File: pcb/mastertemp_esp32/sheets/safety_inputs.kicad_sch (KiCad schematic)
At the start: 0 parts

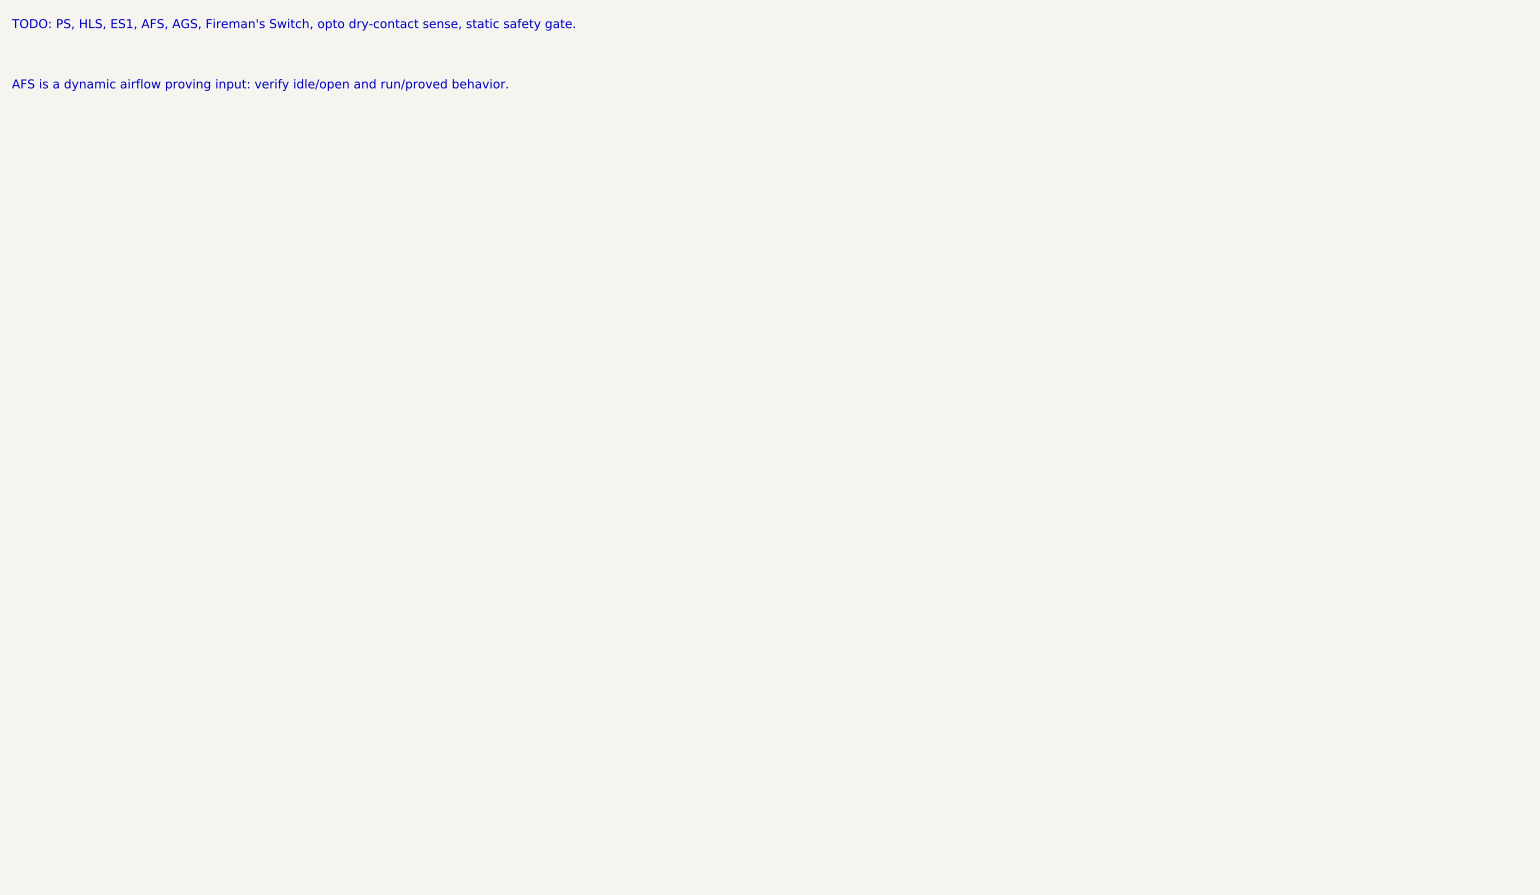
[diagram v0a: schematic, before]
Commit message: Bump
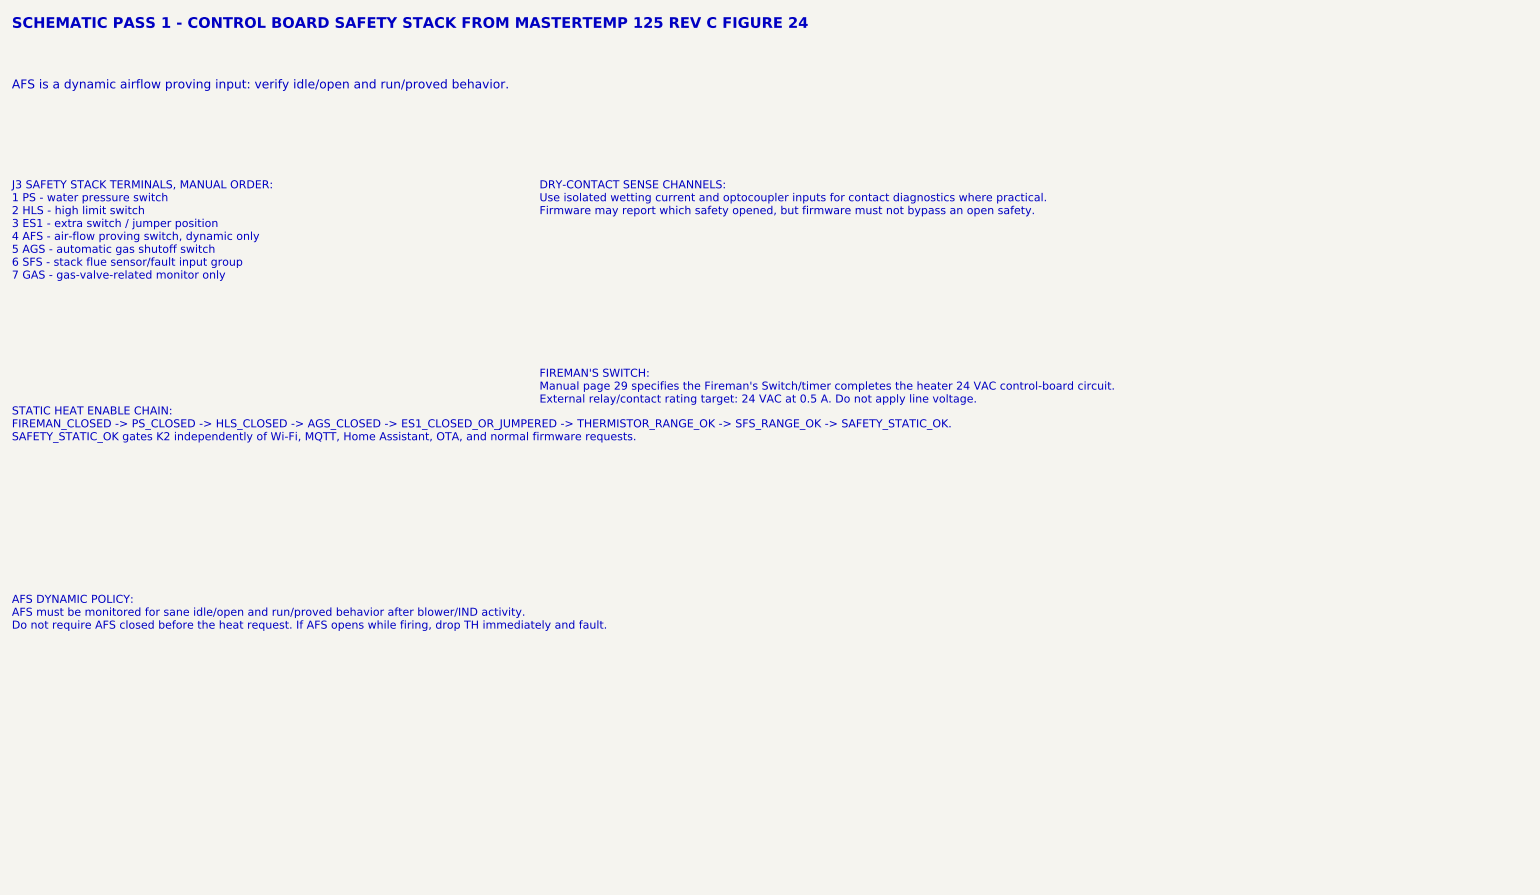
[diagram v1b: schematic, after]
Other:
- note added: "AFS DYNAMIC POLICY: AFS must be monitored for sane idle/open and run/proved behavior after blower/IND activity. Do not require AFS closed before the heat request. If AFS opens while firing, drop TH immediately and fault."
- note added: "DRY-CONTACT SENSE CHANNELS: Use isolated wetting current and optocoupler inputs for contact diagnostics where practical. Firmware may report which safety opened, but firmware must not bypass an open safety."
- note added: "FIREMAN'S SWITCH: Manual page 29 specifies the Fireman's Switch/timer completes the heater 24 VAC control-board circuit. External relay/contact rating target: 24 VAC at 0.5 A. Do not apply line voltage."
- note added: "J3 SAFETY STACK TERMINALS, MANUAL ORDER: 1 PS - water pressure switch 2 HLS - high limit switch 3 ES1 - extra switch / jumper position 4 AFS - air-flow proving switch, dynamic only 5 AGS - automatic gas shutoff switch 6 SFS - stack flue sensor/fault input group 7 GAS - gas-valve-related monitor only"
- note added: "SCHEMATIC PASS 1 - CONTROL BOARD SAFETY STACK FROM MASTERTEMP 125 REV C FIGURE 24"
- note added: "STATIC HEAT ENABLE CHAIN: FIREMAN_CLOSED -> PS_CLOSED -> HLS_CLOSED -> AGS_CLOSED -> ES1_CLOSED_OR_JUMPERED -> THERMISTOR_RANGE_OK -> SFS_RANGE_OK -> SAFETY_STATIC_OK. SAFETY_STATIC_OK gates K2 independently of Wi-Fi, MQTT, Home Assistant, OTA, and normal firmware requests."
- note removed: "TODO: PS, HLS, ES1, AFS, AGS, Fireman's Switch, opto dry-contact sense, static safety gate."
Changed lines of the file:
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@@
     (comment 1 "Safety switches are sensed and participate in hardware gating where appropriate.")
   )
-  (text "TODO: PS, HLS, ES1, AFS, AGS, Fireman's Switch, opto dry-contact sense, static safety gate."
+  (text "SCHEMATIC PASS 1 - CONTROL BOARD SAFETY STACK FROM MASTERTEMP 125 REV C FIGURE 24"
     (at 25.4 25.4 0)
-    (effects (font (size 1.5 1.5)) (justify left bottom))
+    (effects (font (size 1.8 1.8) (bold yes)) (justify left bottom))
   )
   (text "AFS is a dynamic airflow proving input: verify idle/open and run/proved behavior."
@@
     (effects (font (size 1.5 1.5)) (justify left bottom))
   )
+  (text "J3 SAFETY STACK TERMINALS, MANUAL ORDER:\n1 PS - water pressure switch\n2 HLS - high limit switch\n3 ES1 - extra switch / jumper position\n4 AFS - air-flow proving switch, dynamic only\n5 AGS - automatic gas shutoff switch\n6 SFS - stack flue sensor/fault input group\n7 GAS - gas-valve-related monitor only"
+    (at 25.4 50.8 0)
+    (effects (font (size 1.35 1.35)) (justify left top))
+  )
+  (text "STATIC HEAT ENABLE CHAIN:\nFIREMAN_CLOSED -> PS_CLOSED -> HLS_CLOSED -> AGS_CLOSED -> ES1_CLOSED_OR_JUMPERED -> THERMISTOR_RANGE_OK -> SFS_RANGE_OK -> SAFETY_STATIC_OK.\nSAFETY_STATIC_OK gates K2 independently of Wi-Fi, MQTT, Home Assistant, OTA, and normal firmware requests."
+    (at 25.4 88.9 0)
+    (effects (font (size 1.35 1.35)) (justify left top))
+  )
+  (text "AFS DYNAMIC POLICY:\nAFS must be monitored for sane idle/open and run/proved behavior after blower/IND activity.\nDo not require AFS closed before the heat request. If AFS opens while firing, drop TH immediately and fault."
+    (at 25.4 120.65 0)
+    (effects (font (size 1.35 1.35)) (justify left top))
+  )
+  (text "DRY-CONTACT SENSE CHANNELS:\nUse isolated wetting current and optocoupler inputs for contact diagnostics where practical.\nFirmware may report which safety opened, but firmware must not bypass an open safety."
+    (at 114.3 50.8 0)
+    (effects (font (size 1.35 1.35)) (justify left top))
+  )
+  (text "FIREMAN'S SWITCH:\nManual page 29 specifies the Fireman's Switch/timer completes the heater 24 VAC control-board circuit.\nExternal relay/contact rating target: 24 VAC at 0.5 A. Do not apply line voltage."
+    (at 114.3 82.55 0)
+    (effects (font (size 1.35 1.35)) (justify left top))
+  )
   (sheet_instances

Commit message: Make open source.
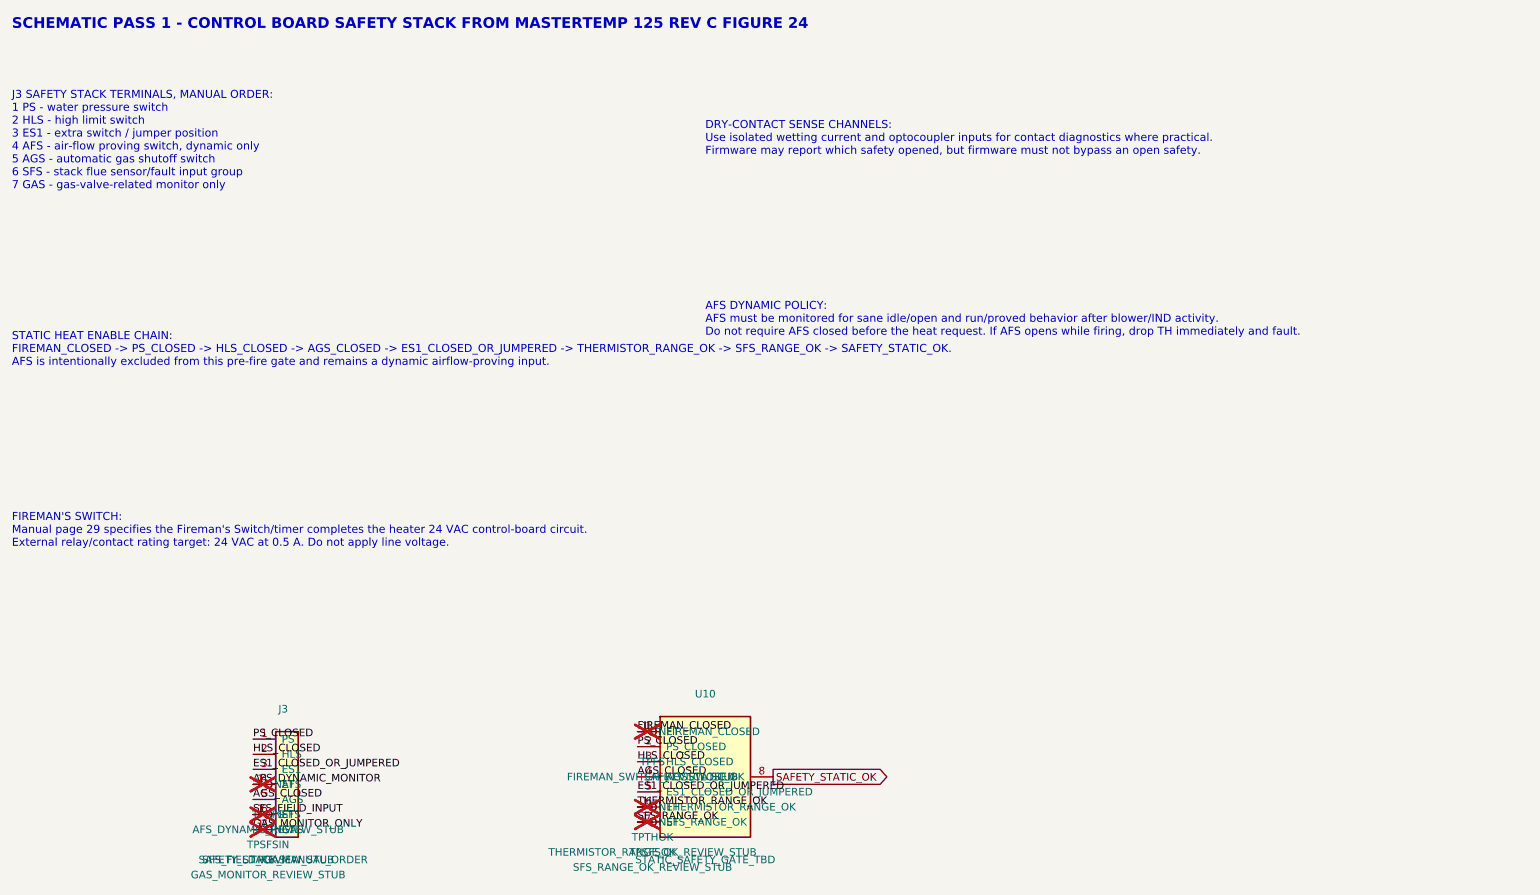
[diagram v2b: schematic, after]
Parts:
- added J3: SAFETY_STACK_MANUAL_ORDER, TerminalBlock_Phoenix:PhoenixContact_MSTBA_2,5_7-G-5,08_1x07_P5.08mm_Horizontal, symbol mastertemp_esp32:SafetyStack_7P
- added TPAFS: AFS_DYNAMIC_REVIEW_STUB, symbol mastertemp_esp32:NetStub_1pin
- added TPFS: FIREMAN_SWITCH_REVIEW_STUB, symbol mastertemp_esp32:NetStub_1pin
- added TPGAS: GAS_MONITOR_REVIEW_STUB, symbol mastertemp_esp32:NetStub_1pin
- added TPSFSIN: SFS_FIELD_REVIEW_STUB, symbol mastertemp_esp32:NetStub_1pin
- added TPSFSOK: SFS_RANGE_OK_REVIEW_STUB, symbol mastertemp_esp32:NetStub_1pin
- added TPTHOK: THERMISTOR_RANGE_OK_REVIEW_STUB, symbol mastertemp_esp32:NetStub_1pin
- added U10: STATIC_SAFETY_GATE_TBD, symbol mastertemp_esp32:StaticSafetyGate
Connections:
- new net AFS_DYNAMIC_MONITOR: J3.4 (AFS), TPAFS.1 (NET)
- new net AGS_CLOSED: J3.5 (AGS), U10.4 (AGS_CLOSED)
- new net ES1_CLOSED_OR_JUMPERED: J3.3 (ES1), U10.5 (ES1_CLOSED_OR_JUMPERED)
- new net FIREMAN_CLOSED: TPFS.1 (NET), U10.1 (FIREMAN_CLOSED)
- new net GAS_MONITOR_ONLY: J3.7 (GAS), TPGAS.1 (NET)
- new net HLS_CLOSED: J3.2 (HLS), U10.3 (HLS_CLOSED)
- new net PS_CLOSED: J3.1 (PS), U10.2 (PS_CLOSED)
- new net SAFETY_STATIC_OK: U10.8 (SAFETY_STATIC_OK)
- new net SFS_FIELD_INPUT: J3.6 (SFS), TPSFSIN.1 (NET)
- new net SFS_RANGE_OK: TPSFSOK.1 (NET), U10.7 (SFS_RANGE_OK)
- new net THERMISTOR_RANGE_OK: TPTHOK.1 (NET), U10.6 (THERMISTOR_RANGE_OK)
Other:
- note added: "STATIC HEAT ENABLE CHAIN: FIREMAN_CLOSED -> PS_CLOSED -> HLS_CLOSED -> AGS_CLOSED -> ES1_CLOSED_OR_JUMPERED -> THERMISTOR_RANGE_OK -> SFS_RANGE_OK -> SAFETY_STATIC_OK. AFS is intentionally excluded from this pre-fire gate and remains a dynamic airflow-proving input."
- note removed: "AFS is a dynamic airflow proving input: verify idle/open and run/proved behavior."
- note removed: "STATIC HEAT ENABLE CHAIN: FIREMAN_CLOSED -> PS_CLOSED -> HLS_CLOSED -> AGS_CLOSED -> ES1_CLOSED_OR_JUMPERED -> THERMISTOR_RANGE_OK -> SFS_RANGE_OK -> SAFETY_STATIC_OK. SAFETY_STATIC_OK gates K2 independently of Wi-Fi, MQTT, Home Assistant, OTA, and normal firmware requests."

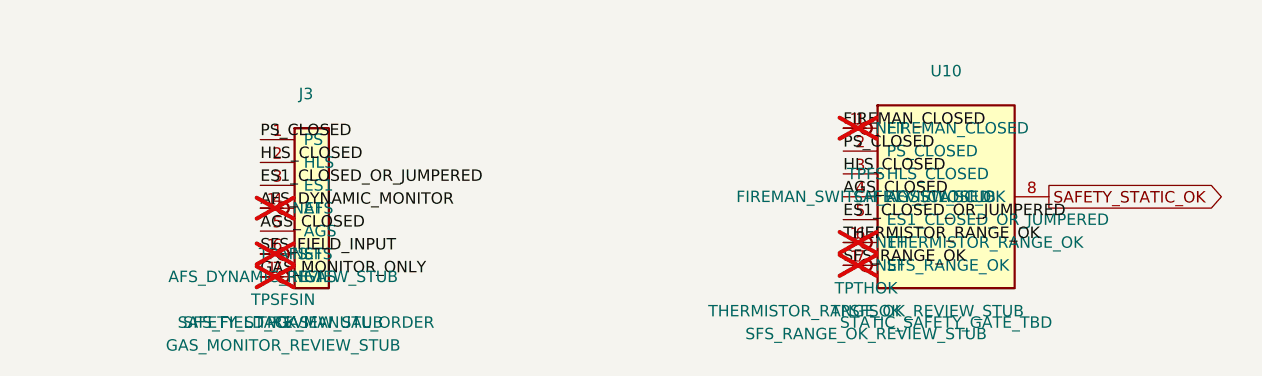
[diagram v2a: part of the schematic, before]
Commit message: AI Gen
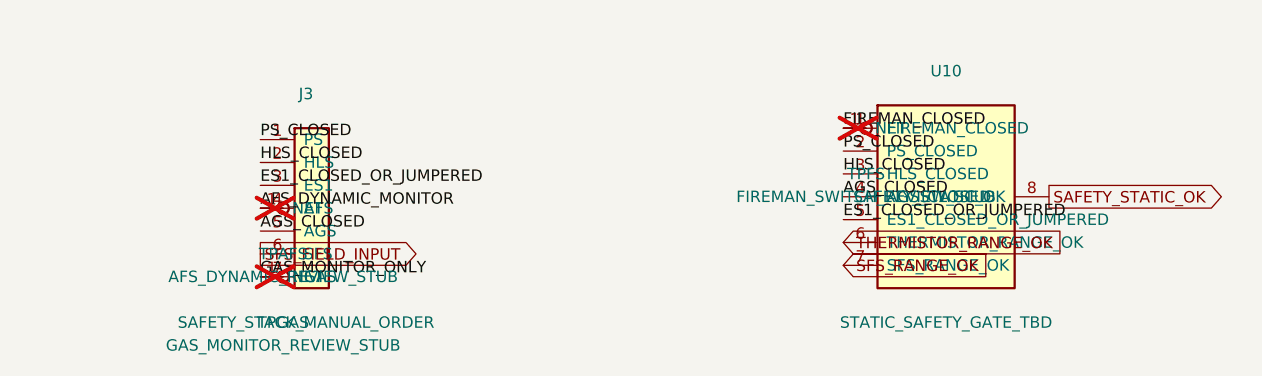
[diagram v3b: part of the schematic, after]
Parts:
- removed TPSFSIN: SFS_FIELD_REVIEW_STUB, symbol mastertemp_esp32:NetStub_1pin
- removed TPSFSOK: SFS_RANGE_OK_REVIEW_STUB, symbol mastertemp_esp32:NetStub_1pin
- removed TPTHOK: THERMISTOR_RANGE_OK_REVIEW_STUB, symbol mastertemp_esp32:NetStub_1pin
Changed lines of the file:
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@@
   (label "AFS_DYNAMIC_MONITOR" (at 66.04 152.4 0) (fields_autoplaced yes) (effects (font (size 1.27 1.27)) (justify left bottom)))
   (label "AGS_CLOSED" (at 66.04 154.94 0) (fields_autoplaced yes) (effects (font (size 1.27 1.27)) (justify left bottom)))
-  (label "SFS_FIELD_INPUT" (at 66.04 157.48 0) (fields_autoplaced yes) (effects (font (size 1.27 1.27)) (justify left bottom)))
+  (global_label "SFS_FIELD_INPUT" (shape output) (at 66.04 157.48 0) (fields_autoplaced yes) (effects (font (size 1.27 1.27)) (justify left bottom)))
   (label "GAS_MONITOR_ONLY" (at 66.04 160.02 0) (fields_autoplaced yes) (effects (font (size 1.27 1.27)) (justify left bottom)))
   (label "FIREMAN_CLOSED" (at 130.81 143.51 0) (fields_autoplaced yes) (effects (font (size 1.27 1.27)) (justify left bottom)))
@@
   (label "AGS_CLOSED" (at 130.81 151.13 0) (fields_autoplaced yes) (effects (font (size 1.27 1.27)) (justify left bottom)))
   (label "ES1_CLOSED_OR_JUMPERED" (at 130.81 153.67 0) (fields_autoplaced yes) (effects (font (size 1.27 1.27)) (justify left bottom)))
-  (label "THERMISTOR_RANGE_OK" (at 130.81 156.21 0) (fields_autoplaced yes) (effects (font (size 1.27 1.27)) (justify left bottom)))
-  (label "SFS_RANGE_OK" (at 130.81 158.75 0) (fields_autoplaced yes) (effects (font (size 1.27 1.27)) (justify left bottom)))
+  (global_label "THERMISTOR_RANGE_OK" (shape input) (at 130.81 156.21 0) (fields_autoplaced yes) (effects (font (size 1.27 1.27)) (justify left bottom)))
+  (global_label "SFS_RANGE_OK" (shape input) (at 130.81 158.75 0) (fields_autoplaced yes) (effects (font (size 1.27 1.27)) (justify left bottom)))
   (global_label "SAFETY_STATIC_OK" (shape output) (at 153.67 151.13 0) (fields_autoplaced yes) (effects (font (size 1.27 1.27)) (justify left bottom)))
   (symbol
@@
     (pin "1")
     (instances (project "mastertemp_esp32" (path "/82ec6d80-25f4-4b98-986b-98eab22f32ad" (reference "TPAFS") (unit 1))))
-  )
-  (symbol
-    (lib_id "mastertemp_esp32:NetStub_1pin")
-    (at 68.58 157.48 0)
-    (unit 1)
-    (exclude_from_sim yes)
-    (in_bom no)
-    (on_board no)
-    (dnp yes)
-    (property "Reference" "TPSFSIN" (at 68.58 162.56 0) (effects (font (size 1.27 1.27))))
-    (property "Value" "SFS_FIELD_REVIEW_STUB" (at 68.58 165.1 0) (effects (font (size 1.27 1.27))))
-    (property "Footprint" "" (at 68.58 157.48 0) (effects (font (size 1.27 1.27)) (hide yes)))
-    (property "Datasheet" "~" (at 68.58 157.48 0) (effects (font (size 1.27 1.27)) (hide yes)))
-    (property "Description" "SFS electrical type and range require field verification" (at 68.58 157.48 0) (effects (font (size 1.27 1.27)) (hide yes)))
-    (pin "1")
-    (instances (project "mastertemp_esp32" (path "/82ec6d80-25f4-4b98-986b-98eab22f32ad" (reference "TPSFSIN") (unit 1))))
   )
   (symbol
@@
     (instances (project "mastertemp_esp32" (path "/82ec6d80-25f4-4b98-986b-98eab22f32ad" (reference "TPFS") (unit 1))))
   )
-  (symbol
-    (lib_id "mastertemp_esp32:NetStub_1pin")
-    (at 133.35 156.21 0)
-    (unit 1)
-    (exclude_from_sim yes)
-    (in_bom no)
-    (on_board no)
-    (dnp yes)
-    (property "Reference" "TPTHOK" (at 133.35 161.29 0) (effects (font (size 1.27 1.27))))
-    (property "Value" "THERMISTOR_RANGE_OK_REVIEW_STUB" (at 133.35 163.83 0) (effects (font (size 1.27 1.27))))
-    (property "Footprint" "" (at 133.35 156.21 0) (effects (font (size 1.27 1.27)) (hide yes)))
-    (property "Datasheet" "~" (at 133.35 156.21 0) (effects (font (size 1.27 1.27)) (hide yes)))
-    (property "Description" "Driven by thermistor comparator in later schematic pass" (at 133.35 156.21 0) (effects (font (size 1.27 1.27)) (hide yes)))
-    (pin "1")
-    (instances (project "mastertemp_esp32" (path "/82ec6d80-25f4-4b98-986b-98eab22f32ad" (reference "TPTHOK") (unit 1))))
-  )
-  (symbol
-    (lib_id "mastertemp_esp32:NetStub_1pin")
-    (at 133.35 158.75 0)
-    (unit 1)
-    (exclude_from_sim yes)
-    (in_bom no)
-    (on_board no)
-    (dnp yes)
-    (property "Reference" "TPSFSOK" (at 133.35 163.83 0) (effects (font (size 1.27 1.27))))
-    (property "Value" "SFS_RANGE_OK_REVIEW_STUB" (at 133.35 166.37 0) (effects (font (size 1.27 1.27))))
-    (property "Footprint" "" (at 133.35 158.75 0) (effects (font (size 1.27 1.27)) (hide yes)))
-    (property "Datasheet" "~" (at 133.35 158.75 0) (effects (font (size 1.27 1.27)) (hide yes)))
-    (property "Description" "Driven by SFS comparator in later schematic pass" (at 133.35 158.75 0) (effects (font (size 1.27 1.27)) (hide yes)))
-    (pin "1")
-    (instances (project "mastertemp_esp32" (path "/82ec6d80-25f4-4b98-986b-98eab22f32ad" (reference "TPSFSOK") (unit 1))))
-  )
   (sheet_instances
